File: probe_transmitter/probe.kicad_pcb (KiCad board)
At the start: 2 copper layers, 28.4 x 28.4 mm, 26 parts, among them Q1 PMST2222, Q2 PMST2222, U1 ATtiny85-20M

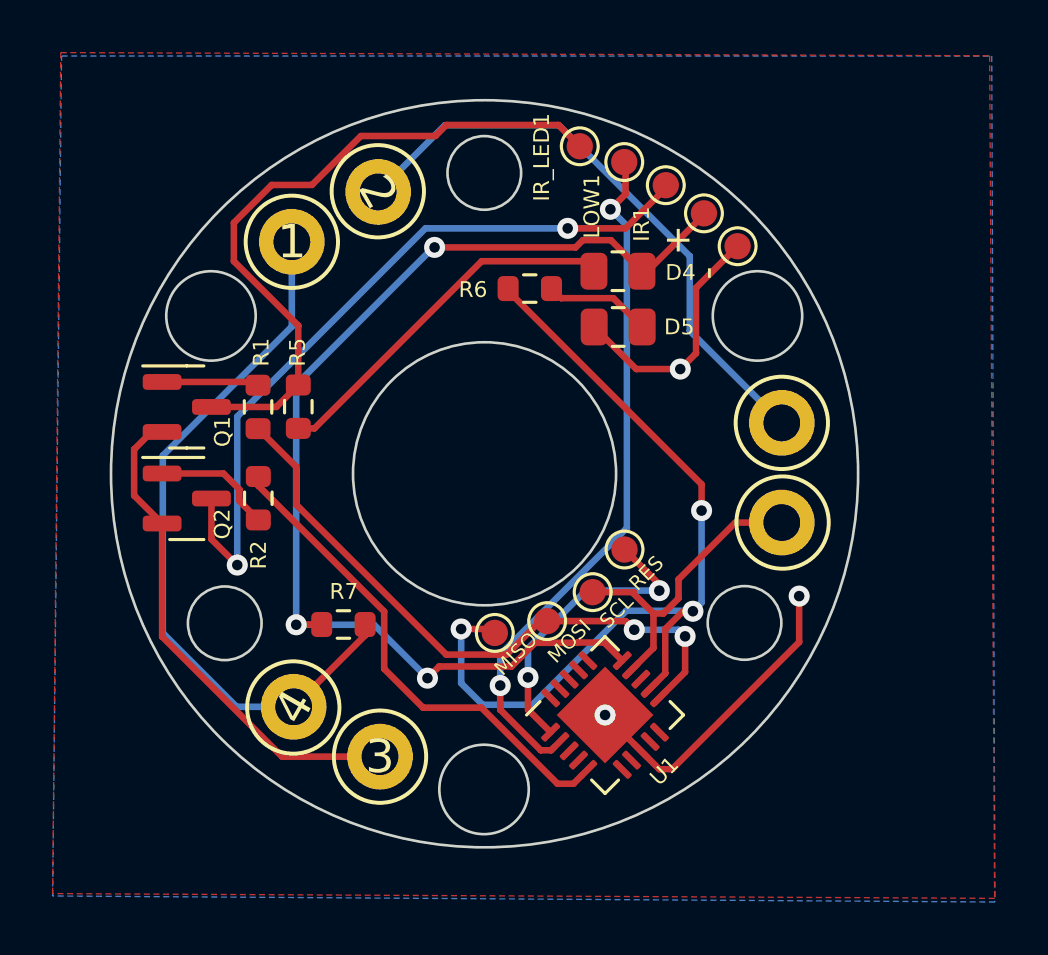
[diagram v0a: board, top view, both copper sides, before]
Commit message: -add new version for transmitter
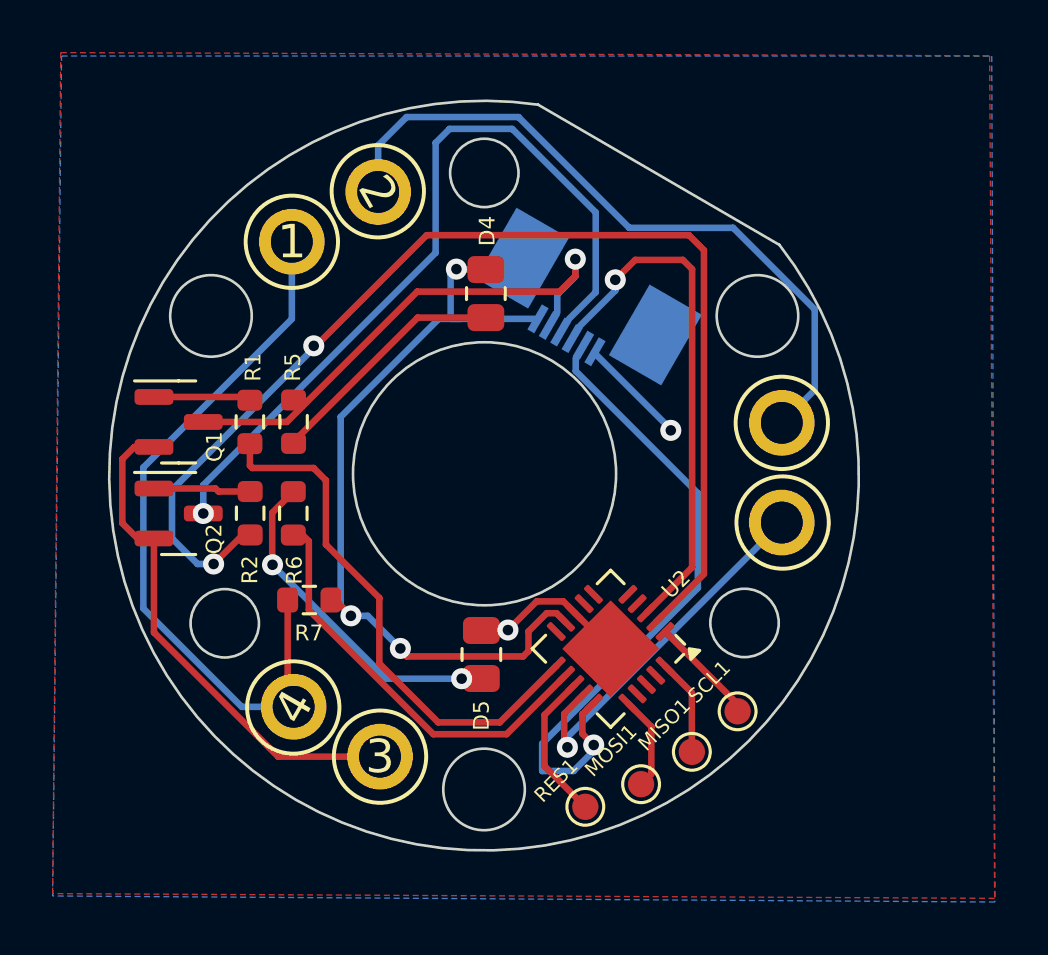
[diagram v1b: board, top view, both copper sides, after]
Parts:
- removed +, -: , TestPoint:TestPoint_Pad_D1.0mm
- removed IR1, IR_LED1: PB4, TestPoint:TestPoint_Pad_D1.0mm
- removed LOW1: PB3, TestPoint:TestPoint_Pad_D1.0mm
- removed U1: ATtiny85-20M, Package_DFN_QFN:QFN-20-1EP_4x4mm_P0.5mm_EP2.6x2.6mm
- added J2: Conn_01x06, Connector_FFC-FPC:TE_0-1734839-6_1x06-1MP_P0.5mm_Horizontal, B.Cu at (103.8, 93.6)
- added U2: ATtiny84-20M, Package_DFN_QFN:QFN-20-1EP_4x4mm_P0.5mm_EP2.6x2.6mm, F.Cu at (104.8, 106.7)
-  : value Touch Probe v1.2 -> Touch Probe v1.4
- moved   16.7 mm to (91.0, 99.8)
- moved D5 13.5 mm to (99.9, 106.9), turned to -90 degrees
- moved R6 12.4 mm to (92.7, 101.5), turned to 90 degrees
- moved RES1 9.89 mm to (103.8, 112.7), turned to 180 degrees
- moved MISO1 8.75 mm to (107.9, 110.6), turned to 180 degrees
- moved MOSI1 7.15 mm to (106.0, 111.8), turned to 180 degrees
- moved SCL1 7.13 mm to (109.6, 109.0), turned to 180 degrees
- moved D4 5.09 mm to (100.0, 93.2), turned to 90 degrees
- moved R7 1.59 mm to (93.3, 104.8), turned to 0 degrees
- moved Q1 0.65 mm to (88.4, 98.0)
- moved Q2 0.65 mm to (88.4, 101.5)
- moved R1 0.65 mm to (91.1, 98.0)
- moved R2 0.65 mm to (91.1, 101.5), turned to 90 degrees
- moved R5 0.60 mm to (92.7, 98.0)
- renumbered MISO to MISO1, MOSI to MOSI1, RES to RES1, SCL to SCL1
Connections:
- MISO1 pad 1: Net-(MISO1-Pad1) -> Net-(U2-PA5)
- MOSI1 pad 1: Net-(MOSI1-Pad1) -> Net-(U2-PA6)
- R1 pad 1: Net-(MOSI1-Pad1) -> Net-(U2-XTAL1/PB0)
- R6 pad 1: Net-(MISO1-Pad1) -> Net-(U2-XTAL2/PB1)
- SCL1 pad 1: /PAD1 -> Net-(U2-PA4)
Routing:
- net Net-(MISO1-Pad1): track 33.6 -> 0.00 mm, vias 3 -> 0
- net Net-(U2-PA3): track 18.8 -> 45.1 mm, vias 0 -> 2
- net Net-(LOW1-Pad1): track 26.0 -> 0.00 mm, vias 2 -> 0
- net Net-(J2-Pin_5): track 0.00 -> 24.5 mm, vias 0 -> 1
- net Net-(MOSI1-Pad1): track 24.4 -> 0.00 mm, vias 2 -> 0
- net Net-(U2-XTAL1/PB0): track 0.00 -> 20.3 mm
- net Net-(J2-Pin_4): track 0.00 -> 19.5 mm, vias 0 -> 1
- net Net-(U2-XTAL2/PB1): track 0.00 -> 16.1 mm
- net +3.3V: track 43.6 -> 31.4 mm
- net GND: track 40.9 -> 28.8 mm, vias 3 -> 2
- net Net-(D5-A): track 4.05 -> 12.1 mm, vias 0 -> 2
- net Net-(J2-Pin_2): track 26.0 -> 19.4 mm, vias 0 -> 1
- net /PAD1: track 63.4 -> 69.8 mm, vias 0 -> 1
- net Net-(U2-~{RESET}/PB3): track 11.6 -> 5.77 mm, vias 2 -> 0
- net Net-(D4-K): track 14.0 -> 9.33 mm
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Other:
- board size 28.4 x 28.4 mm -> 28.5 x 28.5 mm
